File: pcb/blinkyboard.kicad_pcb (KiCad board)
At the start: 2 copper layers, 83 x 78.5 mm, 17 parts, among them U1 4017, U2 NE555P

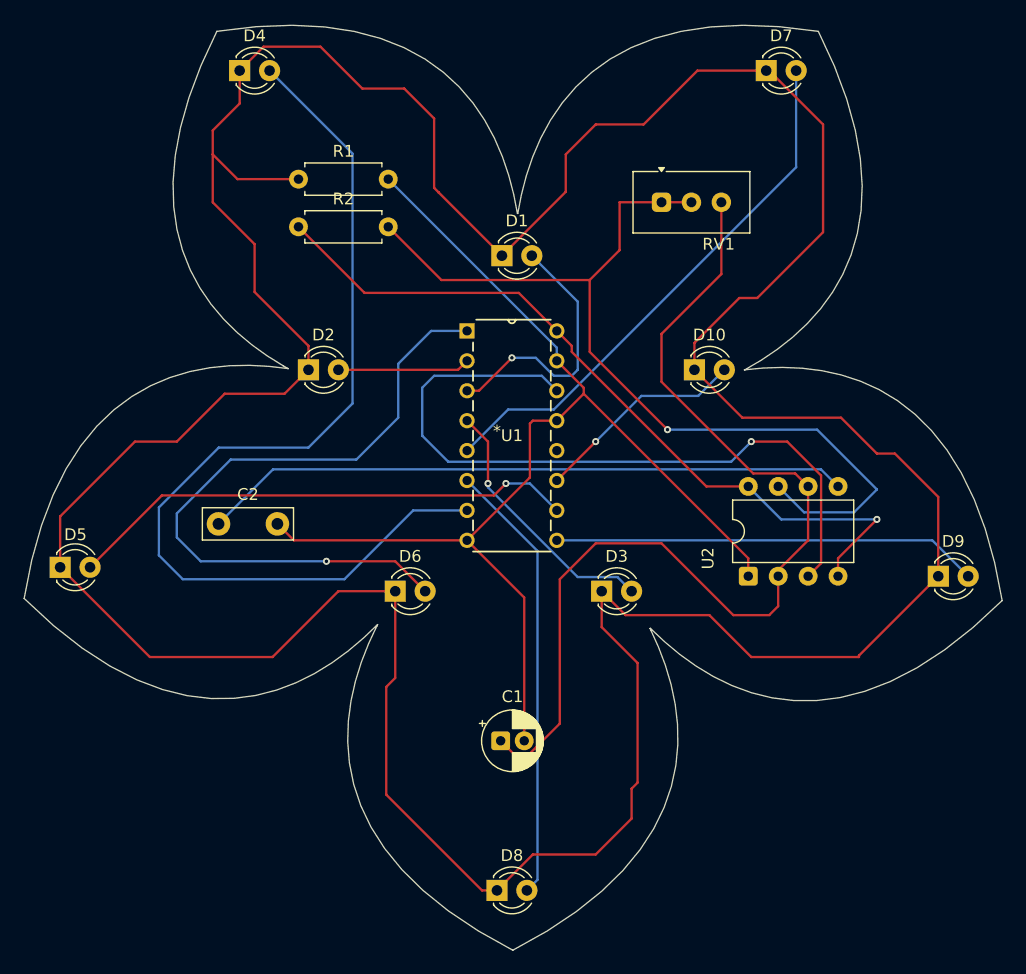
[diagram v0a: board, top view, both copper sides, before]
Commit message: blorp
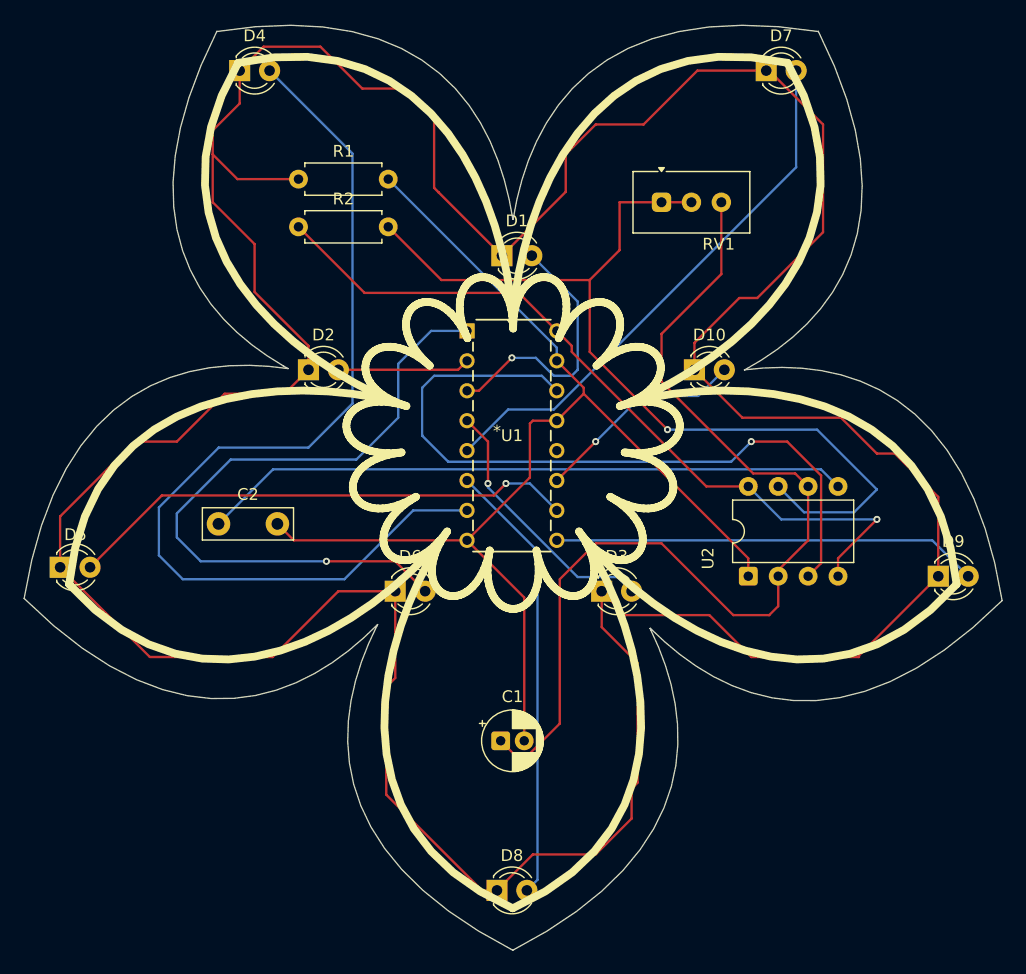
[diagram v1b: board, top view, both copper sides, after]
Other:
- outline, holes or cut-outs redrawn
